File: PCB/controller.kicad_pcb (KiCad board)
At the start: 2 copper layers, 97 x 71.5 mm, 12 parts, among them J1 DC_Air_Pump, J2 ESP32_Joystick_Module, Q2 IRLZ44N, SW1 SW_SPST, U1 LM2596S-5, U3 ESP32-DEVKITC-32D, U4 MPX5010DP

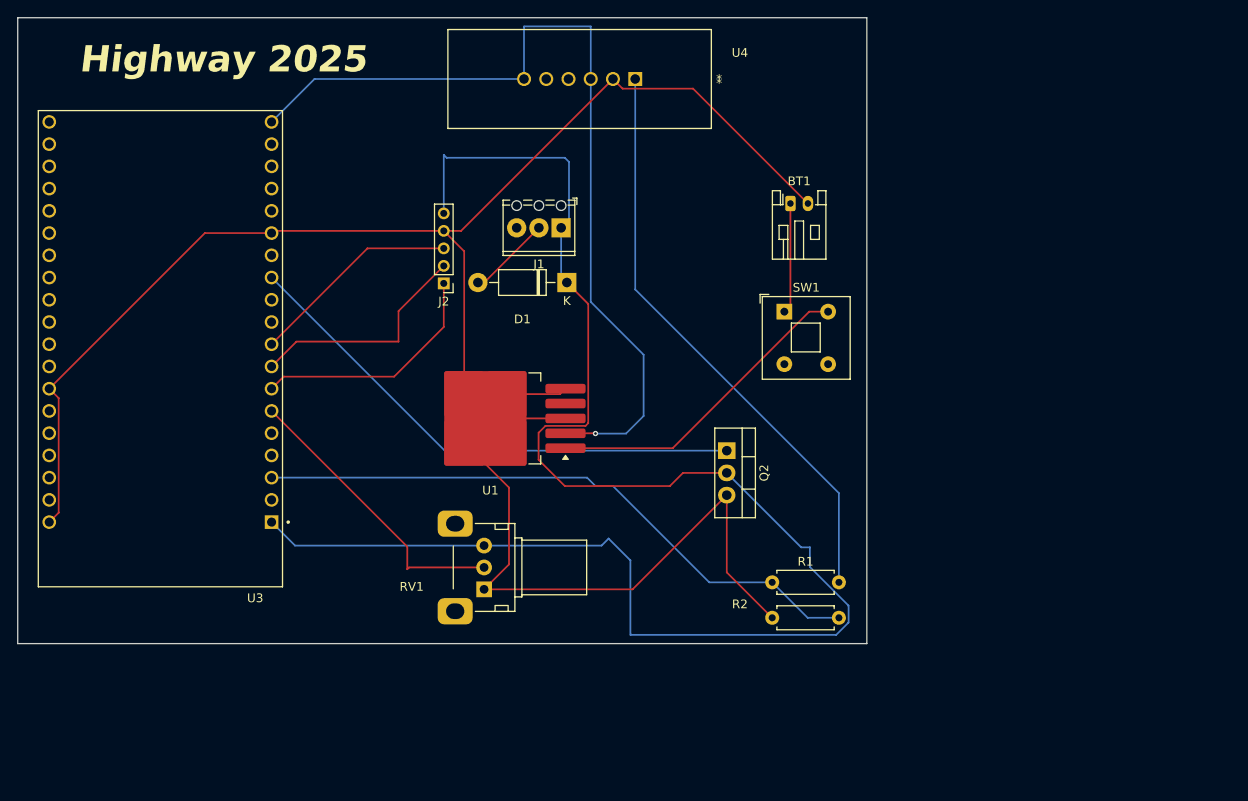
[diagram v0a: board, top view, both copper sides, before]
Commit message: Updated PCB and Production Folders (July 6)
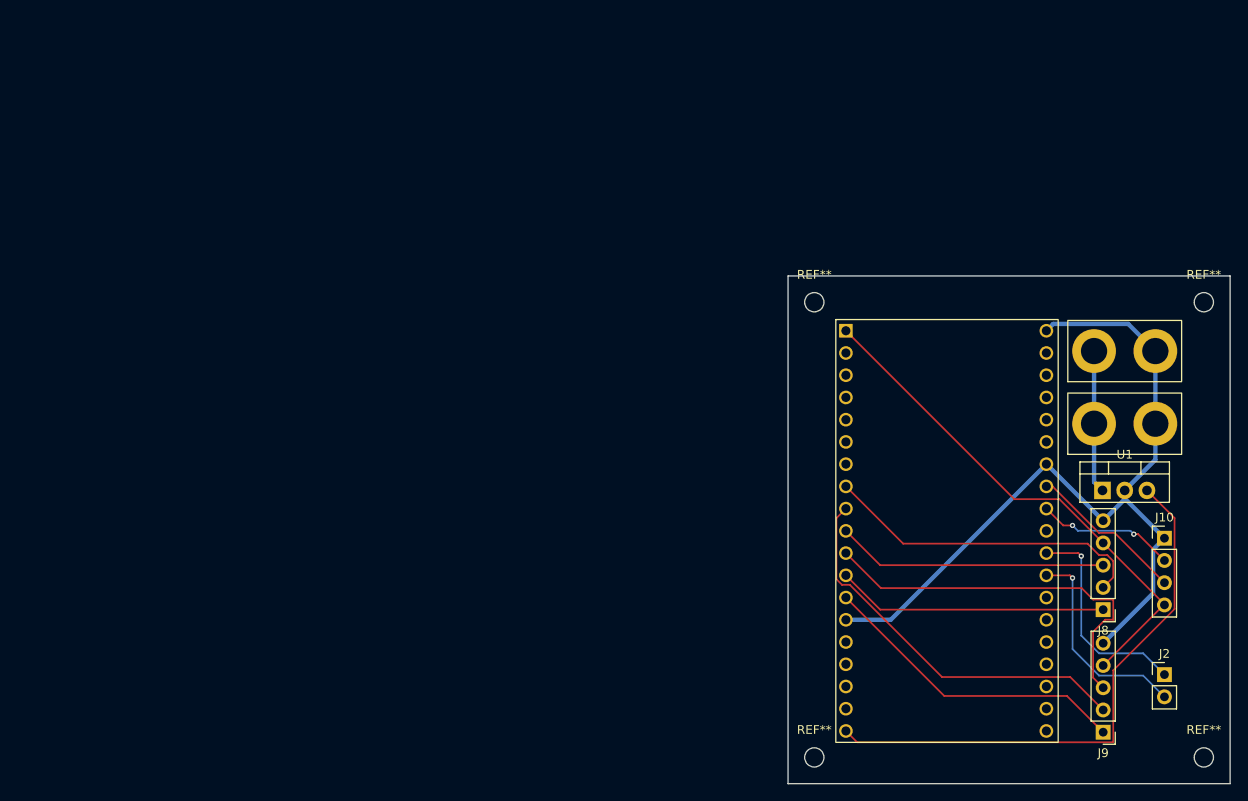
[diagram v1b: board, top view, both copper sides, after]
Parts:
- removed D1: 1N4007, Diode_THT:D_DO-41_SOD81_P10.16mm_Horizontal
- removed Q2: IRLZ44N, Package_TO_SOT_THT:TO-220-3_Vertical
- removed R1: 10k, Resistor_THT:R_Axial_DIN0207_L6.3mm_D2.5mm_P7.62mm_Horizontal
- removed R2: 15k, Resistor_THT:R_Axial_DIN0207_L6.3mm_D2.5mm_P7.62mm_Horizontal
- removed RV1: R_Potentiometer, Potentiometer_THT:Potentiometer_Alps_RK09K_Single_Horizontal
- removed SW1: SW_SPST, Button_Switch_THT:SW_Push_2P1T_Toggle_CK_PVA1xxH1xxxxxxV2
- removed U4: MPX5010DP, controller:MPX5010DP_MOT
- added J10: Pressure Sensor, Connector_PinHeader_2.54mm:PinHeader_1x04_P2.54mm_Vertical, F.Cu at (218.5, 107.5)
- added J8: Joystick 1 (L), Connector_PinHeader_2.54mm:PinHeader_1x05_P2.54mm_Vertical, F.Cu at (211.5, 115.6)
- added J9: Joystick 2 (R), Connector_PinHeader_2.54mm:PinHeader_1x05_P2.54mm_Vertical, F.Cu at (211.5, 129.6)
- added REF**: MountingHole_2.2mm_M2, MountingHole:MountingHole_2.2mm_M2, F.Cu at (178.5, 80.5)
- added REF**: MountingHole_2.2mm_M2, MountingHole:MountingHole_2.2mm_M2, F.Cu at (223.0, 80.5)
- added REF**: MountingHole_2.2mm_M2, MountingHole:MountingHole_2.2mm_M2, F.Cu at (178.5, 132.5)
- added REF**: MountingHole_2.2mm_M2, MountingHole:MountingHole_2.2mm_M2, F.Cu at (223.0, 132.5)
- BT1: footprint Connector_JST:JST_PH_S2B-PH-K_1x02_P2.00mm_Horizontal -> Controller:Battery Connector
- J1: value DC_Air_Pump -> Battery Out; footprint TerminalBlock_Phoenix:TerminalBlock_Phoenix_MPT-0,5-3-2.54_1x03_P2.54mm_Horizontal -> Controller:Battery Connector
- J2: value ESP32_Joystick_Module -> H Bridge In; footprint Connector_PinHeader_2.00mm:PinHeader_1x05_P2.00mm_Vertical -> Connector_PinHeader_2.54mm:PinHeader_1x02_P2.54mm_Vertical
- U1: value LM2596S-5 -> L7805; footprint Package_TO_SOT_SMD:TO-263-5_TabPin3 -> Package_TO_SOT_THT:TO-220-3_Vertical
- U3: footprint ESP32_controller:MODULE_ESP32-DEVKITC-32D -> Controller:ESP32
- moved J2 93.7 mm to (218.5, 123.0), turned to 0 degrees
- moved U3 92.1 mm to (193.4, 107.3), turned to 0 degrees
- moved J1 74.8 mm to (221.0, 94.4), turned to 90 degrees
- moved U1 69.5 mm to (211.4, 102.0), turned to 0 degrees
- moved BT1 48.2 mm to (221.0, 86.1), turned to 90 degrees
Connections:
- BT1 pad 1: Net-(BT1-+) -> /VBAT
- BT1 pad 2: Net-(BT1--) -> GND
- J1 pad 1: Net-(D1-K) -> /VBAT
- J1 pad 2: Net-(D1-A) -> GND
- J2 pad 1: Net-(J2-Pin_1) -> In 1
- J2 pad 2: Net-(J2-Pin_2) -> In 2
- U1 pad 1: Net-(SW1-B) -> /VBAT
- U1 pad 2: Net-(U1-OUT) -> GND
- U1 pad 3: Net-(BT1--) -> +5V
- U3 pad J2-1: Net-(D1-K) -> +3.3V
- U3 pad J2-10: unconnected-(U3-IO26-PadJ2-10) -> X Axis 1
- U3 pad J2-11: unconnected-(U3-IO27-PadJ2-11) -> X Axis 2
- U3 pad J2-12: Net-(Q2-G) -> Button 1
- U3 pad J2-13: unconnected-(U3-IO12-PadJ2-13) -> Button 2
- U3 pad J2-14: Net-(BT1--) -> GND
- U3 pad J2-19: Net-(U1-OUT) -> +5V
- U3 pad J2-3: Net-(U3-SENSOR_VP) -> unconnected-(U3-SENSOR_VP-PadJ2-3)
- U3 pad J2-6: Net-(U3-IO35) -> unconnected-(U3-IO35-PadJ2-6)
- U3 pad J2-7: Net-(J2-Pin_1) -> unconnected-(U3-IO32-PadJ2-7)
- U3 pad J2-8: Net-(J2-Pin_2) -> Y Axis 1
- U3 pad J2-9: Net-(J2-Pin_3) -> Y Axis 2
- U3 pad J3-1: Net-(BT1--) -> GND
- U3 pad J3-11: unconnected-(U3-IO17-PadJ3-11) -> In 1
- U3 pad J3-12: unconnected-(U3-IO16-PadJ3-12) -> In 2
- U3 pad J3-7: Net-(BT1--) -> GND
- U3 pad J3-8: unconnected-(U3-IO19-PadJ3-8) -> Out
- U3 pad J3-9: unconnected-(U3-IO18-PadJ3-9) -> SCK
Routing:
- net Net-(BT1--): track 232.3 -> 0.00 mm
- net Net-(D1-K): track 186.3 -> 0.00 mm
- net Net-(U1-OUT): track 101.3 -> 0.00 mm, vias 1 -> 0
- net GND: track 0.00 -> 97.6 mm
- net Net-(U3-SENSOR_VP): track 71.4 -> 0.00 mm
- net Net-(U4-VOUT): track 67.1 -> 0.00 mm
- net +5V: track 0.00 -> 64.1 mm
- net Net-(Q2-G): track 60.2 -> 0.00 mm
- net +3.3V: track 0.00 -> 59.3 mm
- net Y Axis 2: track 0.00 -> 45.2 mm
- net X Axis 2: track 0.00 -> 44.8 mm
- net Y Axis 1: track 0.00 -> 37.6 mm
- net Net-(SW1-B): track 36.5 -> 0.00 mm
- net Button 2: track 0.00 -> 35.8 mm
- net Net-(U3-IO35): track 33.4 -> 0.00 mm
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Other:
- board size 97 x 71.5 mm -> 50.5 x 58 mm
- board text removed: "Highway 2025"
